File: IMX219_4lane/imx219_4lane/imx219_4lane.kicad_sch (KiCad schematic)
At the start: 25 parts, among them J1 DF37NC-30DS-0.4V, J2 FPC 28 pin connector, Q3 NTZD3154N, U1 AMPM, U2 LM3670MF, U3 AP7331, U4 AP7331

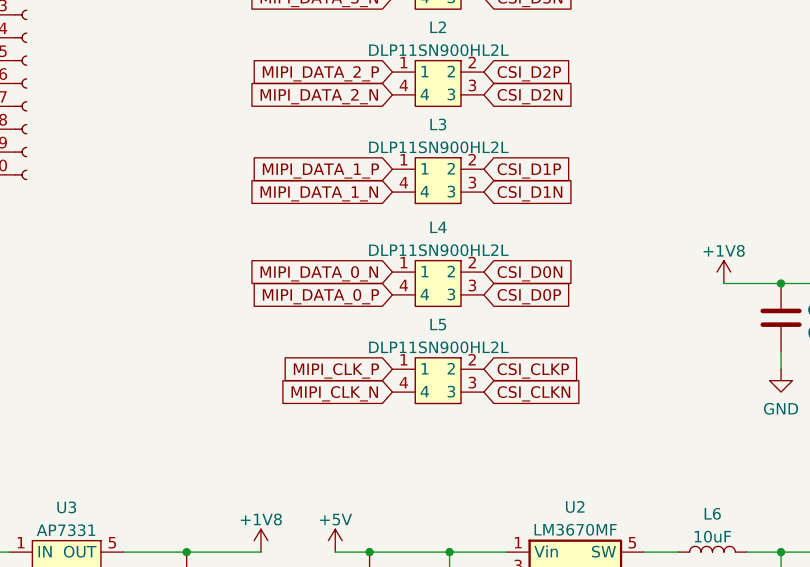
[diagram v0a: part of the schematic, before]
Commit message: prototype routing
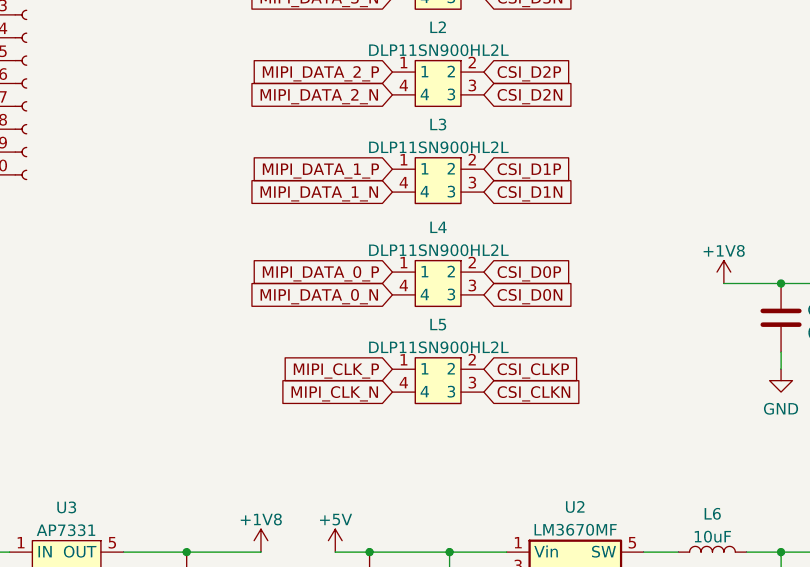
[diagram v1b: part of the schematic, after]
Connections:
- net CSI_D0N: now also L4.3; no longer L4.2
- net CSI_D0P: now also L4.2; no longer L4.3
- net MIPI_DATA_0_N: now also L4.4; no longer L4.1
- net MIPI_DATA_0_P: now also L4.1; no longer L4.4
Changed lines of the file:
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@@
     )
   )
-  (global_label "CSI_D0N" (shape input) (at 99.695 102.87 0) (fields_autoplaced)
-    (effects (font (size 1.27 1.27)) (justify left))
-    (property "Intersheet References" "${INTERSHEET_REFS}" (id 0) (at 109.97 102.7906 0)
-      (effects (font (size 1.27 1.27)) (justify left) hide)
-    )
-  )
-  (global_label "CSI_D0P" (shape input) (at 99.695 105.41 0) (fields_autoplaced)
-    (effects (font (size 1.27 1.27)) (justify left))
-    (property "Intersheet References" "${INTERSHEET_REFS}" (id 0) (at 109.9095 105.3306 0)
+  (global_label "CSI_D0N" (shape input) (at 99.695 105.41 0) (fields_autoplaced)
+    (effects (font (size 1.27 1.27)) (justify left))
+    (property "Intersheet References" "${INTERSHEET_REFS}" (id 0) (at 109.97 105.3306 0)
+      (effects (font (size 1.27 1.27)) (justify left) hide)
+    )
+  )
+  (global_label "CSI_D0P" (shape input) (at 99.695 102.87 0) (fields_autoplaced)
+    (effects (font (size 1.27 1.27)) (justify left))
+    (property "Intersheet References" "${INTERSHEET_REFS}" (id 0) (at 109.9095 102.7906 0)
       (effects (font (size 1.27 1.27)) (justify left) hide)
     )
@@
     )
   )
-  (global_label "MIPI_DATA_0_P" (shape input) (at 89.535 105.41 180) (fields_autoplaced)
-    (effects (font (size 1.27 1.27)) (justify right))
-    (property "Intersheet References" "${INTERSHEET_REFS}" (id 0) (at 73.3938 105.3306 0)
+  (global_label "MIPI_DATA_0_P" (shape input) (at 89.535 102.87 180) (fields_autoplaced)
+    (effects (font (size 1.27 1.27)) (justify right))
+    (property "Intersheet References" "${INTERSHEET_REFS}" (id 0) (at 73.3938 102.7906 0)
       (effects (font (size 1.27 1.27)) (justify right) hide)
     )
@@
     )
   )
-  (global_label "MIPI_DATA_0_N" (shape input) (at 89.535 102.87 180) (fields_autoplaced)
-    (effects (font (size 1.27 1.27)) (justify right))
-    (property "Intersheet References" "${INTERSHEET_REFS}" (id 0) (at 73.3333 102.7906 0)
-      (effects (font (size 1.27 1.27)) (justify right) hide)
-    )
+  (global_label "MIPI_DATA_0_N" (shape input) (at 89.535 105.41 180) (fields_autoplaced)
+    (effects (font (size 1.27 1.27)) (justify right))
+    (property "Intersheet References" "${INTERSHEET_REFS}" (id 0) (at 73.3333 105.3306 0)
+      (effects (font (size 1.27 1.27)) (justify right) hide)
+    )
